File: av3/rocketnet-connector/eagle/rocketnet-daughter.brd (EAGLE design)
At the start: 20.2 x 8 mm, 1 part

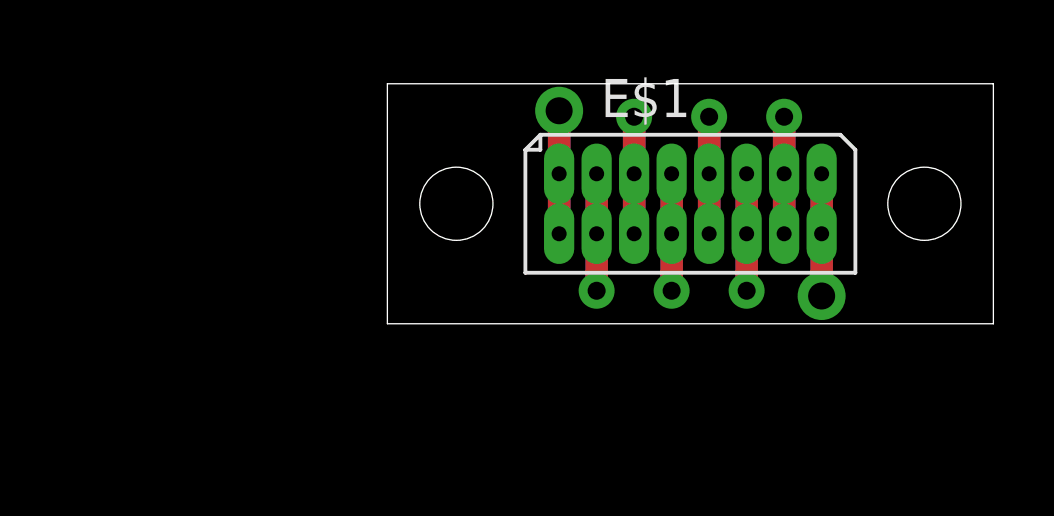
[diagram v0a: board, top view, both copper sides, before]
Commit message: Newer version of rocketnet connector: male on the board side now, female inside custom top. A lot more shallow, but wider now. Let's try it!
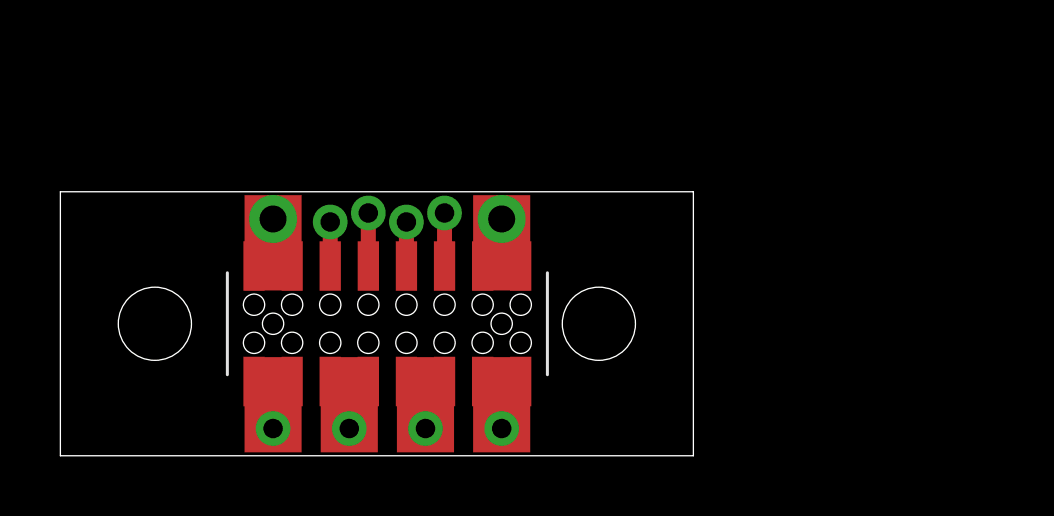
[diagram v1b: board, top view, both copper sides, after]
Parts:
- added E$10, E$11, E$3, E$5, E$6, E$7, E$8, E$9: (no value), rocketnet-connector:26AWG-WIRE
- added E$2: (no value), rocketnet-connector:HARWIN-M50-31508
- added E$4: (no value), rocketnet-connector:22AWG-WIRE
- E$1: device 16-pin-rocketnet-daughter:ROCKETBUS_ROCKETBUS-RECEPTACLE -> rocketnet-connector:22AWG-WIRE
- moved E$1 13.9 mm to (-3.81, 3.49)
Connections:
- removed net AUX1: E$1.AUX1@11
- removed net AUX2: E$1.AUX2@14
- removed net B+: E$1.B+@1, E$1.B+@2
- removed net B-: E$1.B-@15
- removed net RX+: E$1.RX+@7
- removed net RX-: E$1.RX-@10
- removed net TX+: E$1.TX+@3
- removed net TX-: E$1.TX-@6
- new net S$1: E$11.P$1
- new net S$2: E$10.P$1
- new net S$4: E$9.P$1
- new net S$5: E$8.P$1
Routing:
- net B+: track 8.22 -> 0.00 mm, vias 1 -> 0
- net B-: track 8.15 -> 0.00 mm, vias 1 -> 0
- net TX-: track 7.83 -> 0.00 mm
- net RX-: track 7.80 -> 0.00 mm, vias 1 -> 0
- net AUX2: track 7.80 -> 0.00 mm, vias 1 -> 0
- net TX+: track 7.80 -> 0.00 mm, vias 1 -> 0
- net RX+: track 7.80 -> 0.00 mm, vias 1 -> 0
- net AUX1: track 7.80 -> 0.00 mm, vias 1 -> 0
- net S$4: track 0.00 -> 1.95 mm
- net S$5: track 0.00 -> 1.81 mm
- net S$1: track 0.00 -> 1.79 mm
- net S$2: track 0.00 -> 1.49 mm
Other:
- board size 20.2 x 8 mm -> 21.1 x 8.8 mm
- board text added: "AUX3"
- board text added: "AUX4"
- board text added: "TOP VIEW (M50 on top of board)"
- board text removed: "TOP VIEW (JST CONNECTOR FACING UP)"
